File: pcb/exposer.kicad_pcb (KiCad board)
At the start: 2 copper layers, 10 parts, among them IC1 ULN2065B, J1 Conn_01x04_Female, J2 Conn_01x02, SW1 SW_Push, SW2 SW_Push, SW3 SW_Push, SW4 SW_SPST

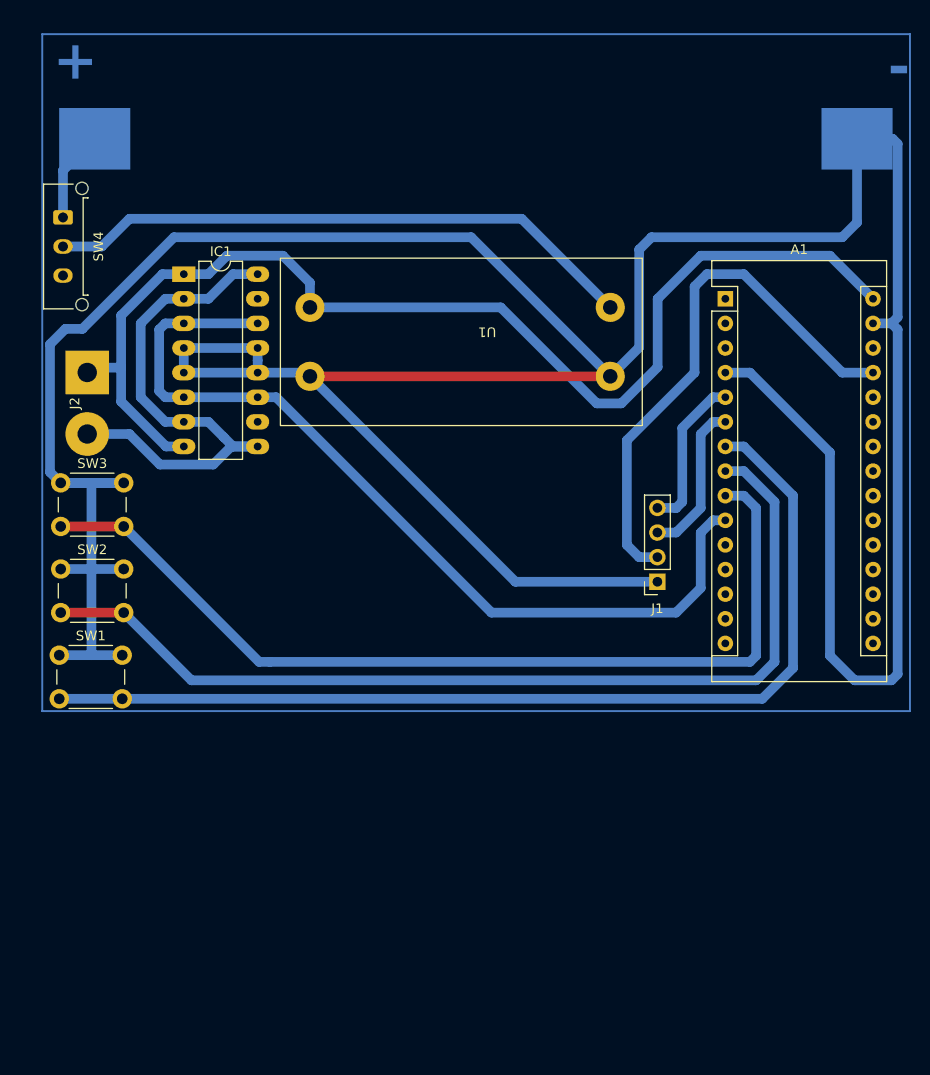
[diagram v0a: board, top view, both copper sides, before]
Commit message: yet another exposer
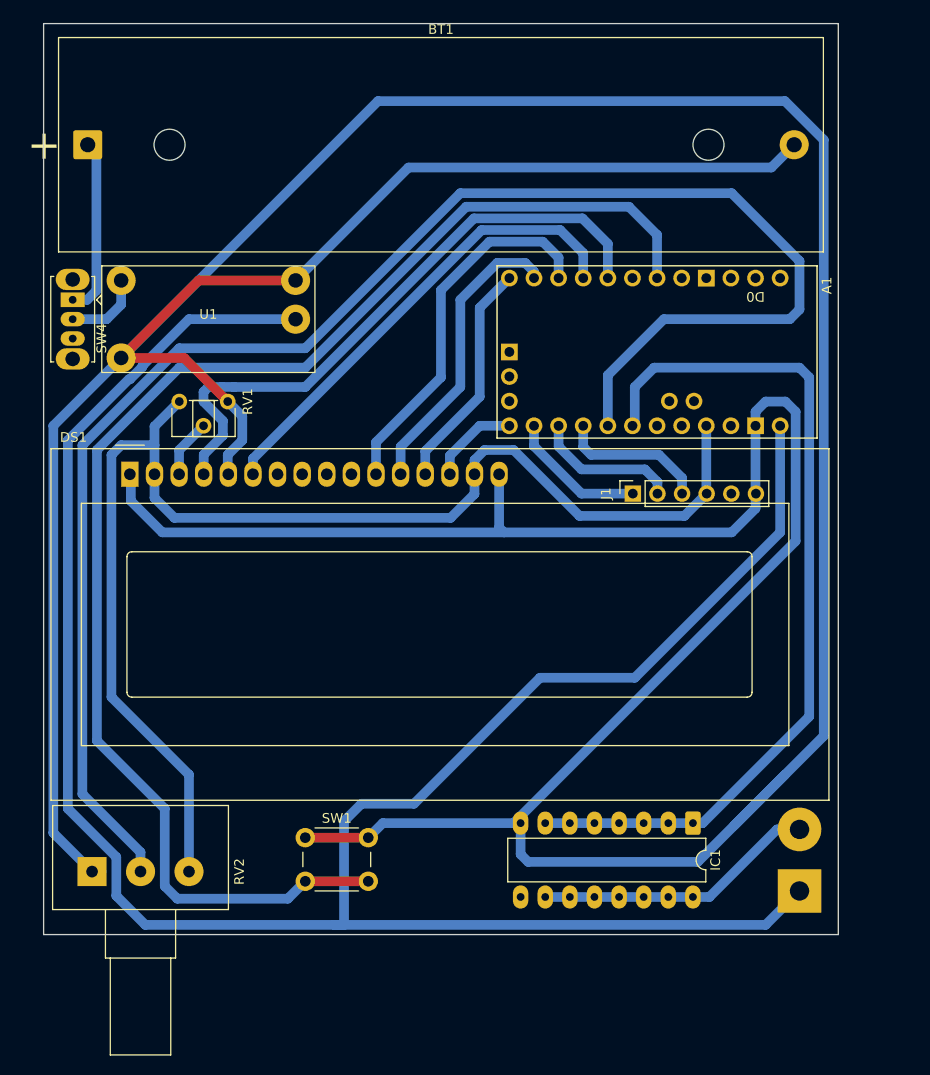
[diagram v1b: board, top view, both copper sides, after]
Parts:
- removed SW2, SW3: SW_Push, Button_Switch_THT:SW_PUSH_6mm_H5mm
- added DS1: WC1602A, Display:WC1602A, F.Cu at (31.9, 67.0)
- added RV1: R_Potentiometer, Potentiometer_THT:Potentiometer_ACP_CA6-H2,5_Horizontal, F.Cu at (42.0, 59.5)
- added RV2: R_Potentiometer, Potentiometer_THT:Potentiometer_Alps_RK163_Single_Horizontal, F.Cu at (28.0, 108.0)
- A1: value Arduino_Nano_v3.x -> Arduino_Pro_Mini_Socket_NoSPH; footprint Module:Arduino_Nano -> arduino-library:Clone_Pro_Mini_Socket_NoSPH
- BT1: footprint Battery:BatteryHolder_Keystone_1042_1x18650 -> Battery:BatteryHolder_MPD_BH-18650-PC; moved to F.Cu
- IC1: value ULN2065B -> ULN2003A
- J1: value Conn_01x04_Female -> Conn_01x06_Socket; footprint Connector_PinSocket_2.54mm:PinSocket_1x04_P2.54mm_Vertical -> Connector_PinSocket_2.54mm:PinSocket_1x06_P2.54mm_Vertical
- SW4: footprint Connector_Molex:Molex_Micro-Fit_3.0_43650-0315_1x03_P3.00mm_Vertical -> Button_Switch_THT:SW_Slide_SPDT_Straight_CK_OS102011MS2Q
- moved J2 90.9 mm to (101.0, 110.0), turned to 90 degrees
- moved IC1 77.3 mm to (90.0, 103.0), turned to -90 degrees
- moved BT1 40.1 mm to (27.6, 33.0)
- moved SW1 31.6 mm to (50.0, 104.5)
- moved U1 28.8 mm to (40.0, 51.0), turned to 0 degrees
- moved J1 9.44 mm to (83.8, 69.0), turned to 90 degrees
- moved A1 8.93 mm to (86.3, 54.4), turned to -90 degrees
- moved SW4 8.56 mm to (26.0, 49.0)
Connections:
- IC1 pad 1: +12V -> Net-(IC1-I1)
- IC1 pad 10: (no net) -> Net-(IC1-O1)
- IC1 pad 11: Net-(A1-D7) -> Net-(IC1-O1)
- IC1 pad 12: GND -> Net-(IC1-O1)
- IC1 pad 13: GND -> Net-(IC1-O1)
- IC1 pad 14: Net-(A1-D7) -> Net-(IC1-O1)
- IC1 pad 15: (no net) -> Net-(IC1-O1)
- IC1 pad 2: Net-(IC1-O1) -> Net-(IC1-I1)
- IC1 pad 3: Net-(A1-D7) -> Net-(IC1-I1)
- IC1 pad 4: GND -> Net-(IC1-I1)
- IC1 pad 5: GND -> Net-(IC1-I1)
- IC1 pad 6: Net-(A1-D7) -> Net-(IC1-I1)
- IC1 pad 7: Net-(IC1-O1) -> Net-(IC1-I1)
- IC1 pad 8: +12V -> GND
- IC1 pad 9: Net-(IC1-O1) -> unconnected-(IC1-COM-Pad9)
- J1 pad 1: GND -> Net-(A1-D11_MOSI)
- J1 pad 2: +5V -> Net-(A1-D12_MISO)
- J1 pad 3: Net-(A1-D3) -> Net-(A1-D13_SCK)
- J1 pad 4: Net-(A1-D2) -> +5V
- SW1 pad 2: Net-(A1-D4) -> Net-(A1-D3_INT1)
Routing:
- net Net-(A1-PadA0): track 0.00 -> 167.0 mm
- net Net-(A1-D3_INT1): track 0.00 -> 144.0 mm
- net GND: track 380.0 -> 521.2 mm
- net +12V: track 121.2 -> 231.0 mm
- net Net-(A1-D4): track 103.9 -> 0.00 mm
- net Net-(A1-D5): track 100.2 -> 0.00 mm
- net Net-(A1-D6): track 96.7 -> 0.00 mm
- net Net-(A1-D7): track 92.0 -> 0.00 mm
- net Net-(IC1-I1): track 0.00 -> 90.1 mm
- net +5V: track 56.4 -> 135.7 mm
- net Net-(DS1-RS): track 0.00 -> 63.9 mm
- net +BATT: track 61.4 -> 8.12 mm
- net Net-(DS1-E): track 0.00 -> 49.0 mm
- net Net-(DS1-D4): track 0.00 -> 38.8 mm
- net Net-(DS1-D5): track 0.00 -> 30.8 mm
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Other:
- board outline added: 82 x 94 mm
- board text removed: "+"
- board text removed: "-"
